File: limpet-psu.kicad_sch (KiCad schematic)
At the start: 16 parts, among them J1 USB_C_Receptacle_HRO_TYPE-C-3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, U1 RT6154AGQW

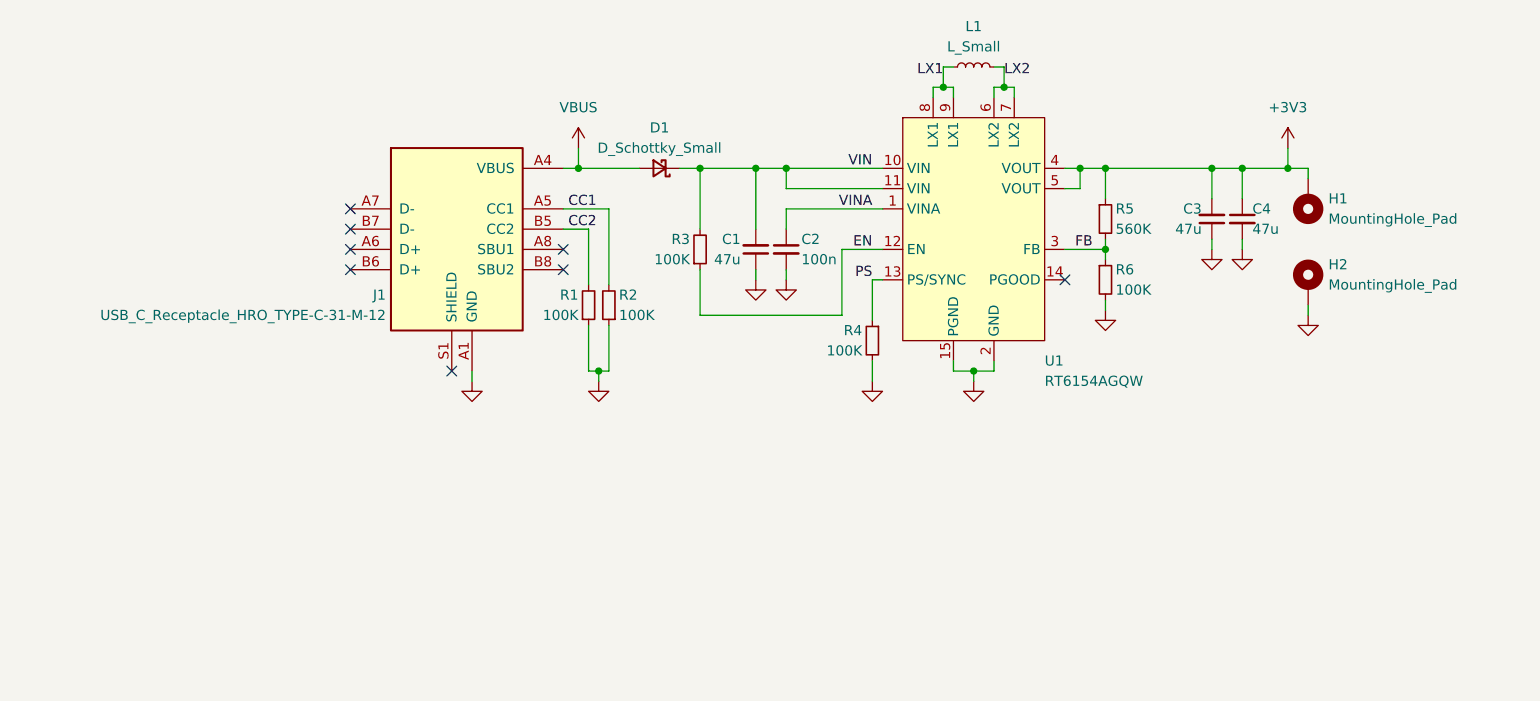
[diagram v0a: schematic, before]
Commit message: 2ndary
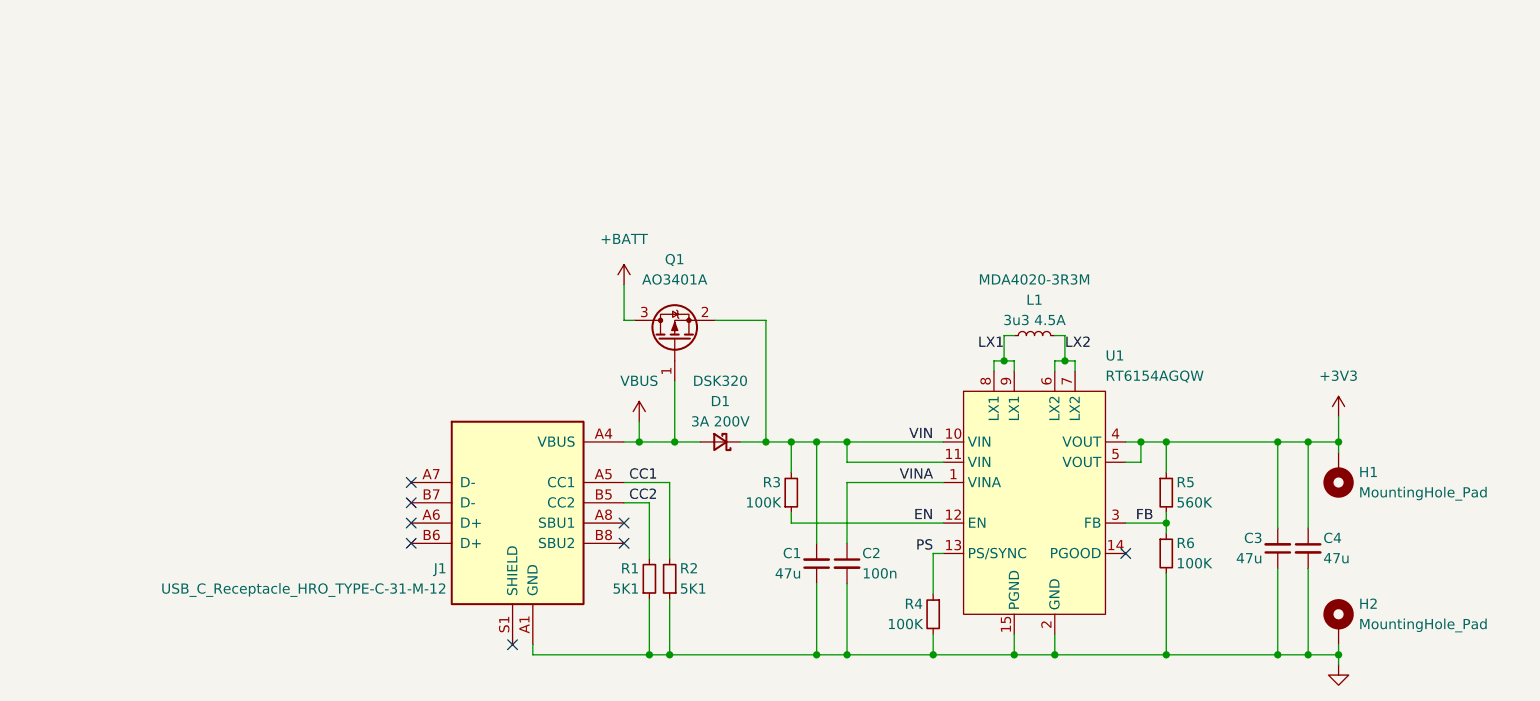
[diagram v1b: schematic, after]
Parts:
- added Q1: AO3401A, Package_TO_SOT_SMD:SOT-23, symbol Transistor_FET:AO3401A
- D1: value D_Schottky_Small -> 3A 200V; Mfr. Part # (none) -> DSK320
- L1: value L_Small -> 3u3 4.5A; Mfr. Part # (none) -> MDA4020-3R3M
- R1, R2: value 100K -> 5K1
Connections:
- net VBUS: now also Q1.1 (G)
- net VIN: now also Q1.2 (S)
- new net +BATT: Q1.3 (D)
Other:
- moved on the sheet: C1, C2, C3, C4, D1, H1, H2, J1, L1, R1, R2, R3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
